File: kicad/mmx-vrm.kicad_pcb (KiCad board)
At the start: 2 copper layers, 39.8 x 46.4 mm, 19 parts, among them J1 Conn_02x15_Row_Letter_First, SW1 SW_DIP_x03, U1 LM2596S, U2 LM2596S

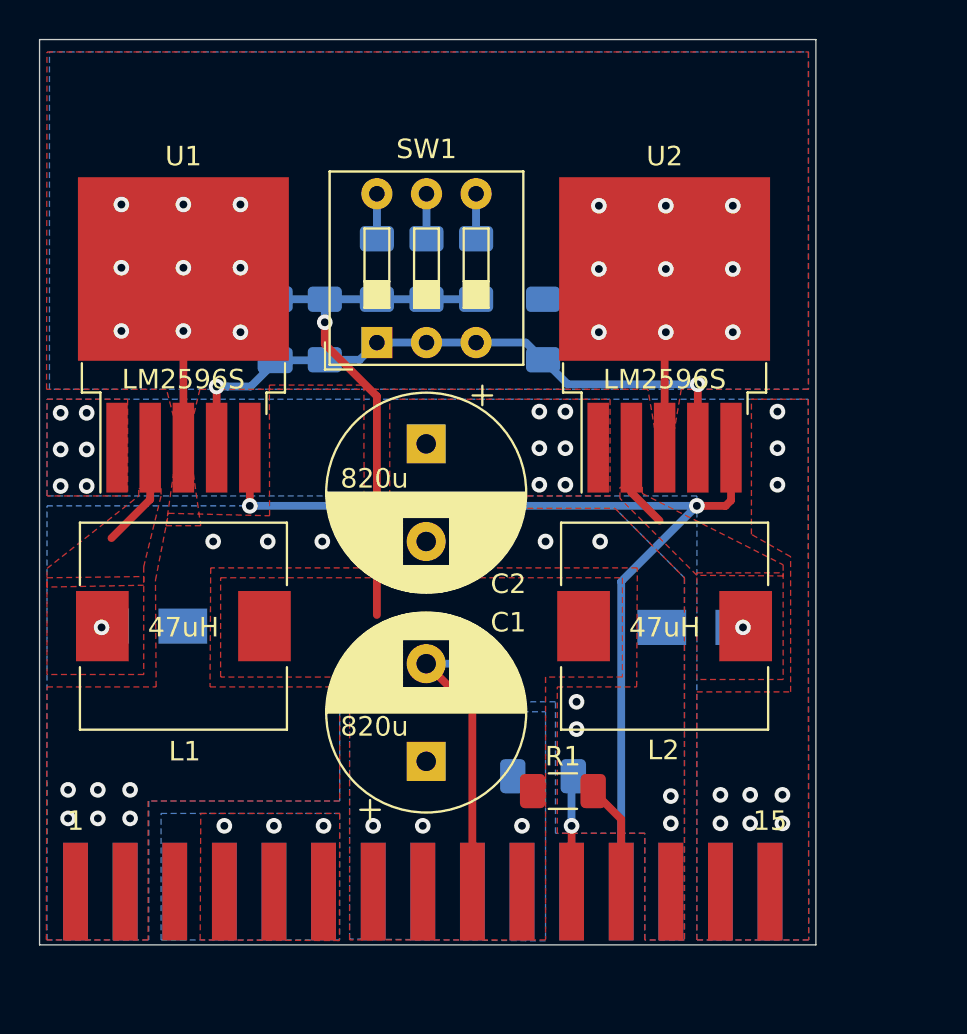
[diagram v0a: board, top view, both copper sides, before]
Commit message: First raw version
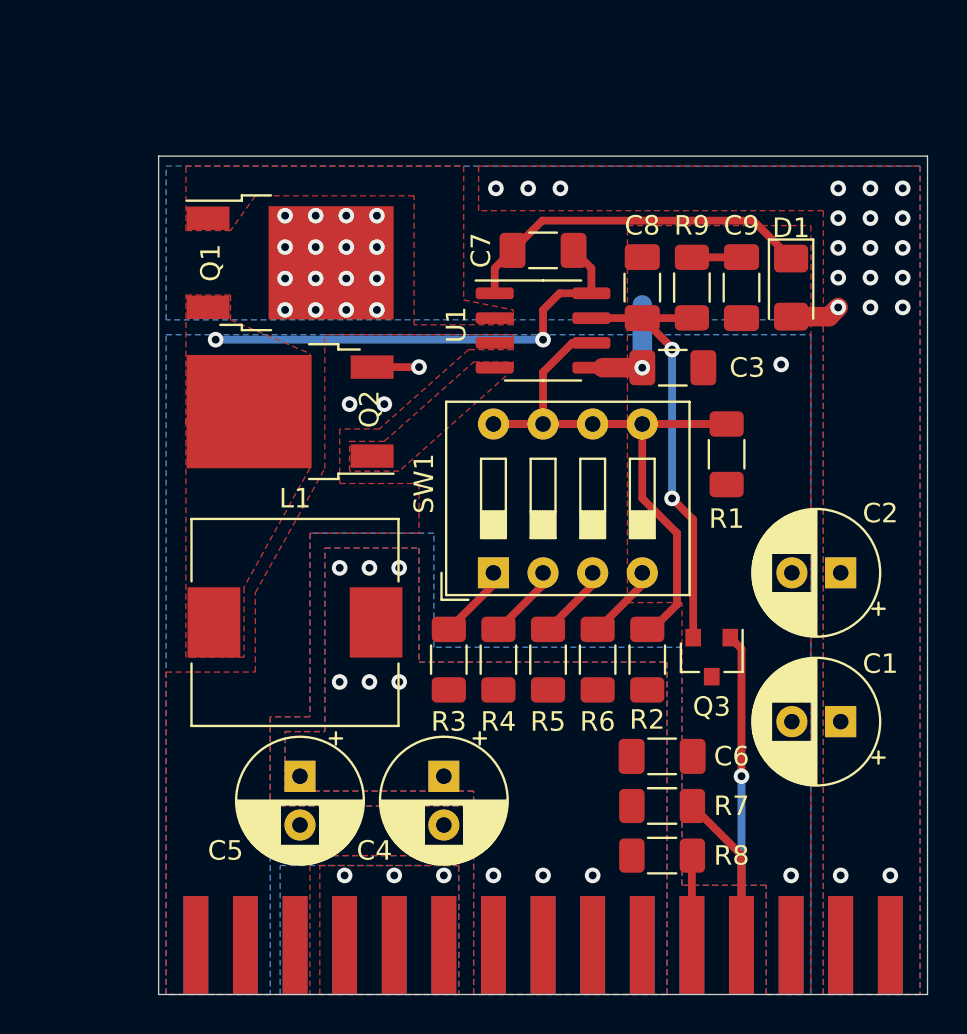
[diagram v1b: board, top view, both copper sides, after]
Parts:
- removed D2: 1N5820, Diode_SMD:D_SMA
- removed L2: 47uH, Inductor_SMD:L_10.4x10.4_H4.8
- removed REF**: OSHW-Logo2_9.8x8mm_SilkScreen, Symbol:OSHW-Logo2_9.8x8mm_SilkScreen
- removed U2: LM2596S, Package_TO_SOT_SMD:TO-263-5_TabPin3
- added C4: 1mF, Capacitor_THT:CP_Radial_D6.3mm_P2.50mm, F.Cu at (133.3, 96.8)
- added C5: 1mF, Capacitor_THT:CP_Radial_D6.3mm_P2.50mm, F.Cu at (126.0, 96.8)
- added C6: 0.1u, Capacitor_SMD:C_1206_3216Metric_Pad1.33x1.80mm_HandSolder, F.Cu at (144.5, 95.8)
- added C7: 0.1u, Capacitor_SMD:C_1206_3216Metric_Pad1.33x1.80mm_HandSolder, F.Cu at (138.4, 69.8)
- added C8: C, Capacitor_SMD:C_1206_3216Metric_Pad1.33x1.80mm_HandSolder, F.Cu at (143.5, 71.8)
- added C9: C, Capacitor_SMD:C_1206_3216Metric_Pad1.33x1.80mm_HandSolder, F.Cu at (148.6, 71.8)
- added Q1: Q_NMOS_GDS, Package_TO_SOT_SMD:TO-252-2, F.Cu at (125.5, 70.5)
- added Q2: Q_NMOS_GDS, Package_TO_SOT_SMD:TO-252-2, F.Cu at (125.5, 78.1)
- added Q3: Q_NPN_BCE, Package_TO_SOT_SMD:SOT-23, F.Cu at (147.1, 90.7)
- added R8: 1K, Resistor_SMD:R_1206_3216Metric_Pad1.30x1.75mm_HandSolder, F.Cu at (144.5, 100.8)
- added R9: R, Resistor_SMD:R_1206_3216Metric_Pad1.30x1.75mm_HandSolder, F.Cu at (146.1, 71.8)
- C1, C2: value 820u -> 1mF; footprint Capacitor_THT:CP_Radial_D10.0mm_P5.00mm -> Capacitor_THT:CP_Radial_D6.3mm_P2.50mm
- C3: value 10nF -> 0.1u; moved to F.Cu
- D1: value 1N5820 -> D; footprint Diode_SMD:D_SMA -> Diode_SMD:D_1206_3216Metric_Pad1.42x1.75mm_HandSolder; moved to F.Cu
- R1: value 0 -> 1K
- R2: value 1K -> 3K; moved to F.Cu
- R3: value 9.1K -> 21K; moved to F.Cu
- R4: value 6.3K -> 15K; moved to F.Cu
- R5: value 3K -> 6,3K; moved to F.Cu
- R6: value 1.6K -> 3K; moved to F.Cu
- R7: value 1K -> 0; moved to F.Cu
- SW1: footprint Button_Switch_THT:SW_DIP_SPSTx03_Slide_9.78x9.8mm_W7.62mm_P2.54mm -> Button_Switch_THT:SW_DIP_SPSTx04_Slide_9.78x12.34mm_W7.62mm_P2.54mm
- U1: value LM2596S -> NCP1579; footprint Package_TO_SOT_SMD:TO-263-5_TabPin3 -> Package_SO:SOIC-8_3.9x4.9mm_P1.27mm
- moved D1 37.4 mm to (151.1, 71.8), turned to 270 degrees
- moved R7 25.1 mm to (144.5, 98.3), turned to 180 degrees
- moved C2 22.2 mm to (153.7, 86.4), turned to 180 degrees
- moved R6 21.9 mm to (141.2, 90.8), turned to 90 degrees
- moved C1 21.3 mm to (153.7, 94.0), turned to 180 degrees
- moved C3 20.5 mm to (145.1, 75.9), turned to 0 degrees
- moved R3 20.3 mm to (133.6, 90.8)
- moved R4 20.3 mm to (136.1, 90.8)
- moved R5 20.3 mm to (138.7, 90.8)
- moved R1 19.2 mm to (147.8, 80.3), turned to 270 degrees
- moved U1 18.4 mm to (138.4, 74.0), turned to 0 degrees
- moved SW1 13.2 mm to (135.9, 86.4)
- moved R2 8.01 mm to (143.8, 90.8), turned to 90 degrees
- moved J1 6.74 mm to (120.7, 102.9)
- moved L1 5.72 mm to (125.7, 88.9)
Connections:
- C1 pad 1: VCORE -> +5V
- C3 pad 1: VCORE -> +5V
- C3 pad 2: FB -> GND
- D1 pad 1: Net-(D1-Pad1) -> Net-(C7-Pad1)
- D1 pad 2: GND -> +5V
- J1 pad a9: GND -> (no net)
- L1 pad 1: Net-(D1-Pad1) -> Net-(C7-Pad2)
- R1 pad 1: SENSE -> FB
- R1 pad 2: VCORE -> GND
- R2 pad 1: PWRGOOD -> VCORE
- R2 pad 2: VCORE -> FB
- R6 pad 2: FB -> Net-(R6-Pad2)
- R7 pad 1: FB -> SENSE
- R7 pad 2: GND -> VCORE
- SW1 pad 1: FB -> Net-(R3-Pad2)
- SW1 pad 2: FB -> Net-(R4-Pad2)
- SW1 pad 3: FB -> Net-(R5-Pad2)
- SW1 pad 4: Net-(R5-Pad2) -> Net-(R6-Pad2)
- SW1 pad 5: Net-(R4-Pad2) -> FB
- SW1 pad 6: Net-(R3-Pad2) -> FB
- U1 pad 1: +5V -> Net-(C7-Pad1)
- U1 pad 2: Net-(D1-Pad1) -> Net-(Q1-Pad1)
- U1 pad 4: FB -> Net-(Q2-Pad1)
- U1 pad 5: DISABLE -> +5V
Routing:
- net DISABLE: track 50.5 -> 16.0 mm, vias 2 -> 1
- net VCORE: track 27.6 -> 0.00 mm, vias 4 -> 9
- net GND: track 27.1 -> 2.40 mm, vias 34 -> 5
- net Net-(C7-Pad2): track 0.00 -> 23.7 mm, vias 0 -> 2
- net Net-(C8-Pad1): track 0.00 -> 22.6 mm, vias 0 -> 2
- net Net-(C7-Pad1): track 0.00 -> 18.3 mm
- net +5V: track 0.00 -> 7.56 mm, vias 21 -> 37
- net Net-(D2-Pad1): track 6.38 -> 0.00 mm, vias 1 -> 0
- net Net-(D1-Pad1): track 5.45 -> 0.00 mm, vias 1 -> 0
- net FB: track 32.8 -> 37.8 mm, vias 2 -> 0
- net Net-(R6-Pad2): track 0.00 -> 3.84 mm
- net SENSE: track 4.47 -> 8.15 mm
- net Net-(C9-Pad1): track 0.00 -> 2.55 mm
- net Net-(R5-Pad2): track 2.30 -> 3.84 mm
- net Net-(R4-Pad2): track 2.30 -> 3.84 mm
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- added copper zone on F.Cu, net Net-(C7-Pad2)
- added copper zone on F.Cu, net Net-(Q1-Pad1)
- added copper zone on F.Cu, net Net-(Q2-Pad1)
- removed copper zone on F.Cu, net Net-(D1-Pad1)
- removed copper zone on F.Cu, net Net-(D2-Pad1)
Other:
- board size 39.8 x 46.4 mm -> 39.4 x 42.9 mm
- net class Power added: clearance 0.2, trace_width 1, via_dia 0.8, via_drill 0.4
- board text removed: "1"
- board text removed: "15"
- board text removed: "MMX-VRM by Necroware"
- board text removed: "SW1 Settings: 000: 3.2V 100: 2.9V 010: 2.8V 110: 2.6V 001: 2.5V 101: 2.4V 011: 2.3V 111: 2.2V"
- board text removed: "rev 0.2"
